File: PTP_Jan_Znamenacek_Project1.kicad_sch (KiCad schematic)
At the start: 25 parts, among them J1 Screw_Terminal_01x02, U2 LM2574N-5, U7 NE555P

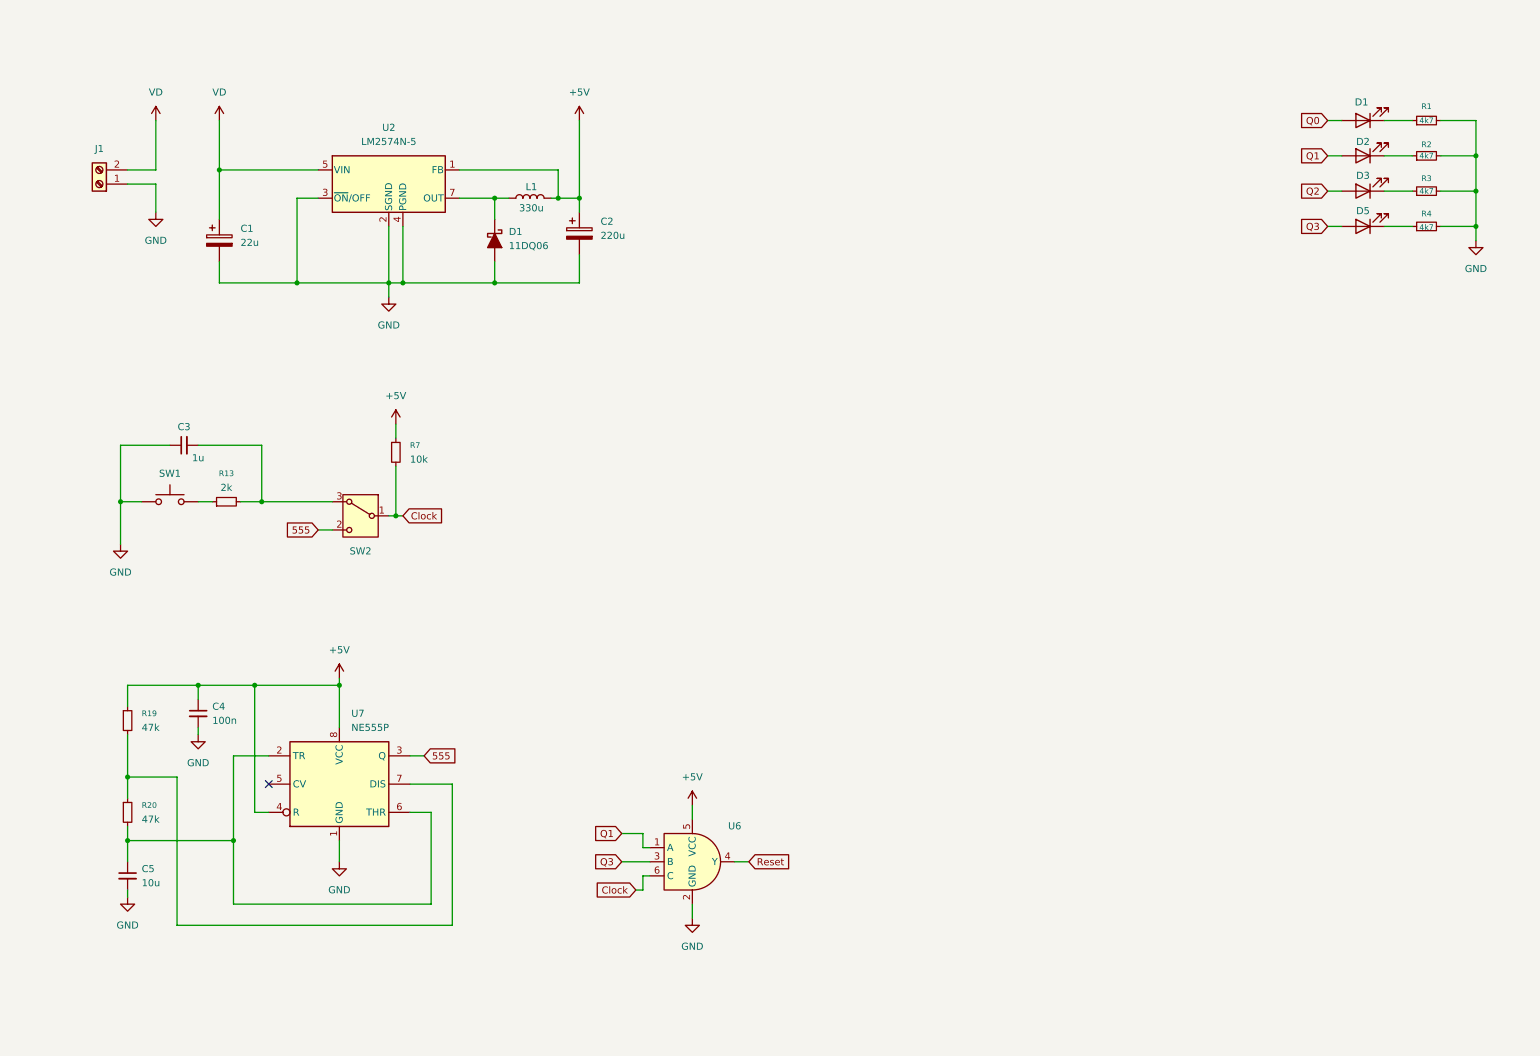
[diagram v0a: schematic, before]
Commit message: LV_4
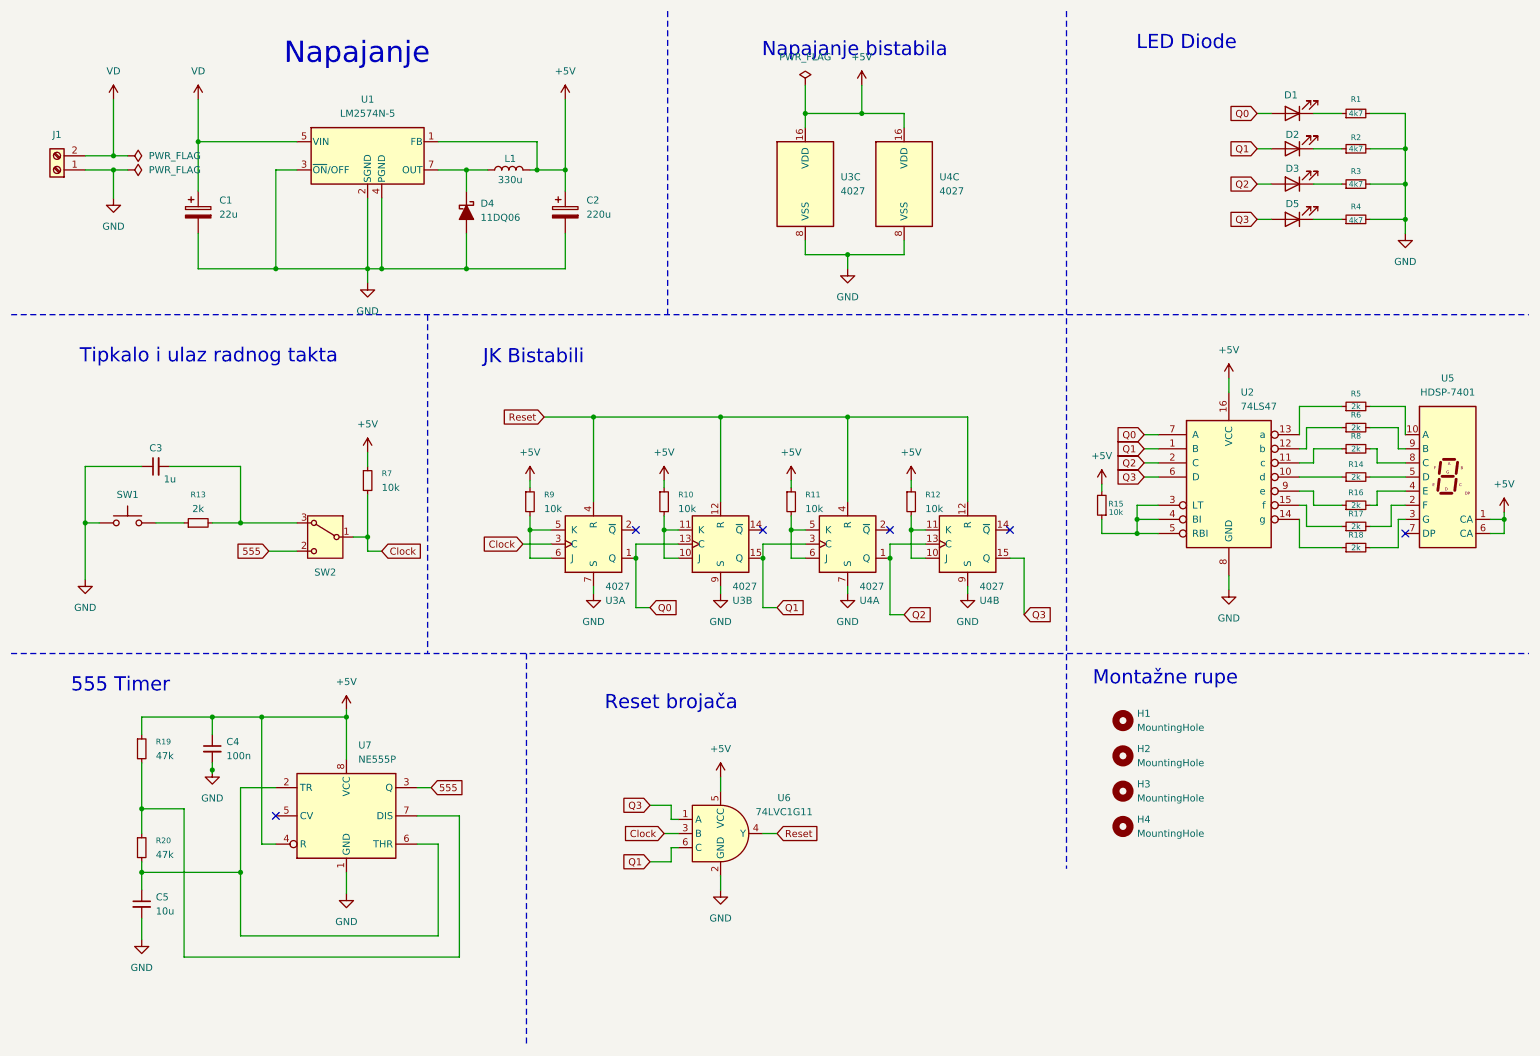
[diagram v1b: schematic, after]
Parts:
- added H1, H2, H3, H4: MountingHole, MountingHole:MountingHole_5.5mm, symbol Mechanical:MountingHole
- added R10, R11, R12, R15, R9: 10k, symbol Device:R_Small
- added R14, R16, R17, R18, R5, R6, R8: 2k, symbol Device:R_Small
- added U2: 74LS47, symbol 74xx:74LS47
- added U3, U4: 4027, symbol 4xxx:4027
- added U5: HDSP-7401, Display_7Segment:HDSP-7401, symbol Display_Character:HDSP-7401
- C1: footprint (none) -> Capacitor_THT:CP_Radial_D5.0mm_P2.00mm; Manufacturer (none) -> AISHI; Manufacturer Part Number (none) -> EWH1EM220D11OT
- C2: footprint (none) -> Capacitor_THT:CP_Radial_D5.0mm_P2.00mm; Manufacturer (none) -> SAMWHA; Manufacturer Part Number (none) -> RD1A227M05011BB
- C3: footprint (none) -> Capacitor_SMD:C_1206_3216Metric_Pad1.33x1.80mm_HandSolder; Manufacturer (none) -> SAMSUNG; Manufacturer Part Number (none) -> CL31B105KBHNNNE
- C4: footprint (none) -> Capacitor_SMD:C_1206_3216Metric_Pad1.33x1.80mm_HandSolder; Manufacturer (none) -> SAMSUNG; Manufacturer Part Number (none) -> CL31B104KBCNNNC
- C5: footprint (none) -> Capacitor_SMD:C_1206_3216Metric_Pad1.33x1.80mm_HandSolder; Manufacturer (none) -> SAMSUNG; Manufacturer Part Number (none) -> CL31A106KBHNNNE
- D1, D2, D3, D5: footprint (none) -> LED_THT:LED_D5.0mm
- D4: renamed from D1; footprint (none) -> Diode_THT:D_DO-41_SOD81_P12.70mm_Horizontal; Manufacturer (none) -> SMC DIODE SOLUTIONS; Manufacturer Part Number (none) -> 11DQ06TA
- J1: footprint (none) -> TerminalBlock_MetzConnect:TerminalBlock_MetzConnect_Type011_RT05502HBLC_1x02_P5.00mm_Horizontal; Manufacturer (none) -> DEGSON ELECTRONICS; Manufacturer Part Number (none) -> DG301-5.0-02P-12-00A(H)
- L1: footprint (none) -> Inductor_THT:L_Radial_D7.2mm_P3.00mm_Murata_1700; Manufacturer (none) -> FERROCORE; Manufacturer Part Number (none) -> COIL0608-0.33
- R1, R2, R3, R4: footprint (none) -> Resistor_THT:R_Axial_DIN0207_L6.3mm_D2.5mm_P10.16mm_Horizontal
- U6: value ~ -> 74LVC1G11
- renumbered U2 to U1
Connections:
- net +5V: now also R10.1, R11.1, R12.1, R15.2, R9.1, U2.16 (VCC), U3.16 (VDD), U4.16 (VDD), U5.1 (CA), U5.6 (CA)
- net Clock: now also U6.3 (B), U3.3 (C); no longer U6.6 (C)
- net GND: now also U2.8 (GND), U3.7 (S), U3.8 (VSS), U3.9 (S), U4.7 (S), U4.8 (VSS), U4.9 (S)
- net Q0: now also U2.7 (A), U3.1 (Q), U3.13 (C)
- net Q1: now also U6.6 (C), U2.1 (B), U3.15 (Q), U4.3 (C); no longer U6.1 (A)
- net Q2: now also U2.2 (C), U4.1 (Q), U4.13 (C)
- net Q3: now also U6.1 (A), U2.6 (D), U4.15 (Q); no longer U6.3 (B)
- net Reset: now also U3.12 (R), U3.4 (R), U4.12 (R), U4.4 (R)
- new net: R11.2, U4.5 (K), U4.6 (J)
- new net: R14.1, U2.10 (d)
- new net: R8.1, U2.11 (c)
- new net: R6.1, U2.12 (b)
- new net: R5.1, U2.13 (a)
- new net: R18.1, U2.14 (g)
- new net: R17.1, U2.15 (f)
- new net: R15.1, U2.3 (LT), U2.4 (BI), U2.5 (RBI)
- new net: R16.1, U2.9 (e)
- new net: R10.2, U3.10 (J), U3.11 (K)
- new net: R12.2, U4.10 (J), U4.11 (K)
- new net: R8.2, U5.8 (C)
- new net: R16.2, U5.4 (E)
- new net: R18.2, U5.3 (G)
- new net: R9.2, U3.5 (K), U3.6 (J)
- new net: R5.2, U5.10 (A)
- new net: R17.2, U5.2 (F)
- new net: R14.2, U5.5 (D)
- new net: R6.2, U5.9 (B)
- no-connect marks 1 -> 6
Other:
- note added: "555 Timer"
- note added: "JK Bistabili"
- note added: "LED Diode"
- note added: "Montažne rupe"
- note added: "Napajanje"
- note added: "Napajanje bistabila"
- note added: "Reset brojača"
- note added: "Tipkalo i ulaz radnog takta"
- moved on the sheet: C1, C2, C3, C4, C5, D1, D2, D3, D4, D5, J1, L1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

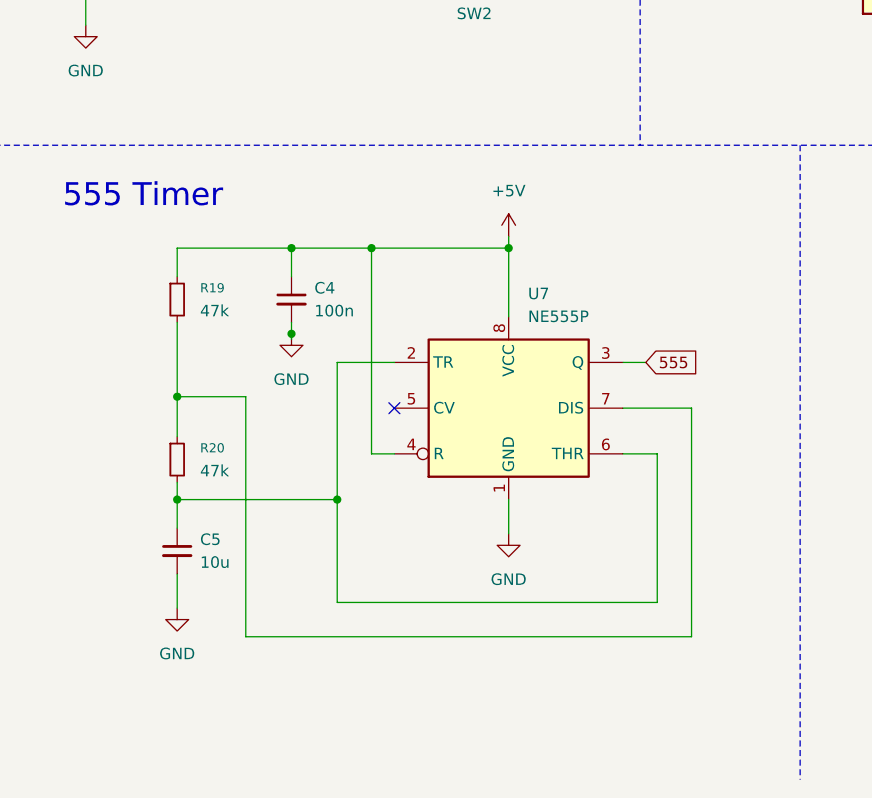
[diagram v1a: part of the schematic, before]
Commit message: PCB Pocetak
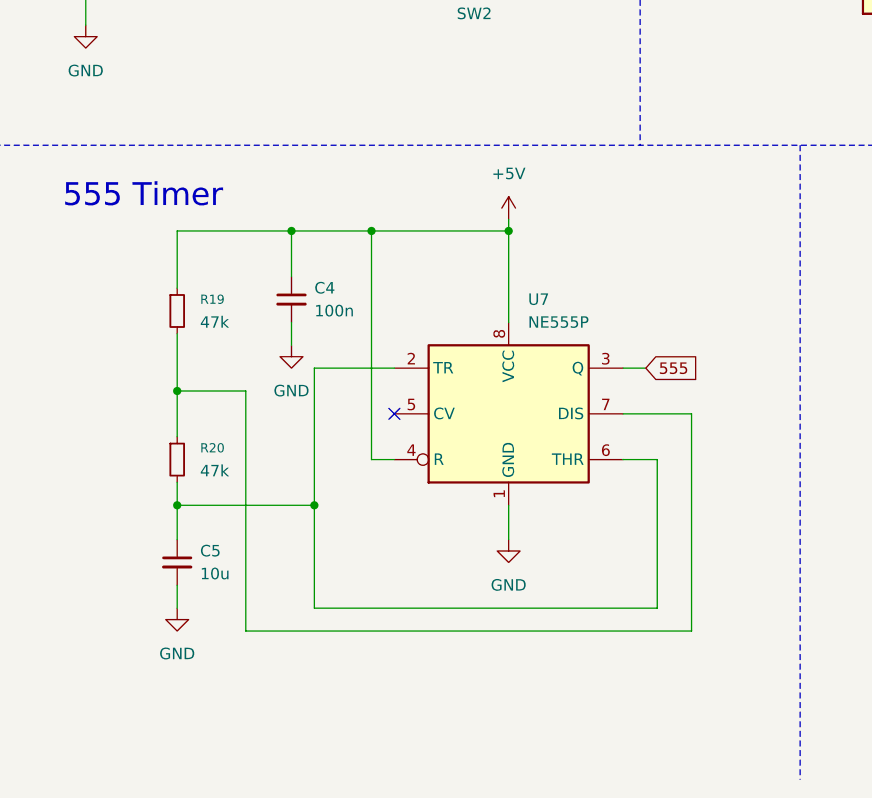
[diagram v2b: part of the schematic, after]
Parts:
- R10, R11, R12, R13, R14, R15, R16, R17, R18, R19, R20, R5, R6, R7, R8, R9: footprint (none) -> Resistor_SMD:R_1206_3216Metric_Pad1.30x1.75mm_HandSolder
- SW1: footprint (none) -> Button_Switch_THT:SW_PUSH_6mm_H4.3mm
- SW2: footprint (none) -> Button_Switch_THT:SW_Slide_SPDT_Straight_CK_OS102011MS2Q
- U2, U3, U4: footprint (none) -> Package_DIP:DIP-16_W7.62mm_Socket_LongPads
- U6: footprint (none) -> Package_TO_SOT_SMD:SOT-23-6
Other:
- moved on the sheet: C5, R19, U7
